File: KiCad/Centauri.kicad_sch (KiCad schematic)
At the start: 137 parts, among them U1 Raspberry_Pi_Pico

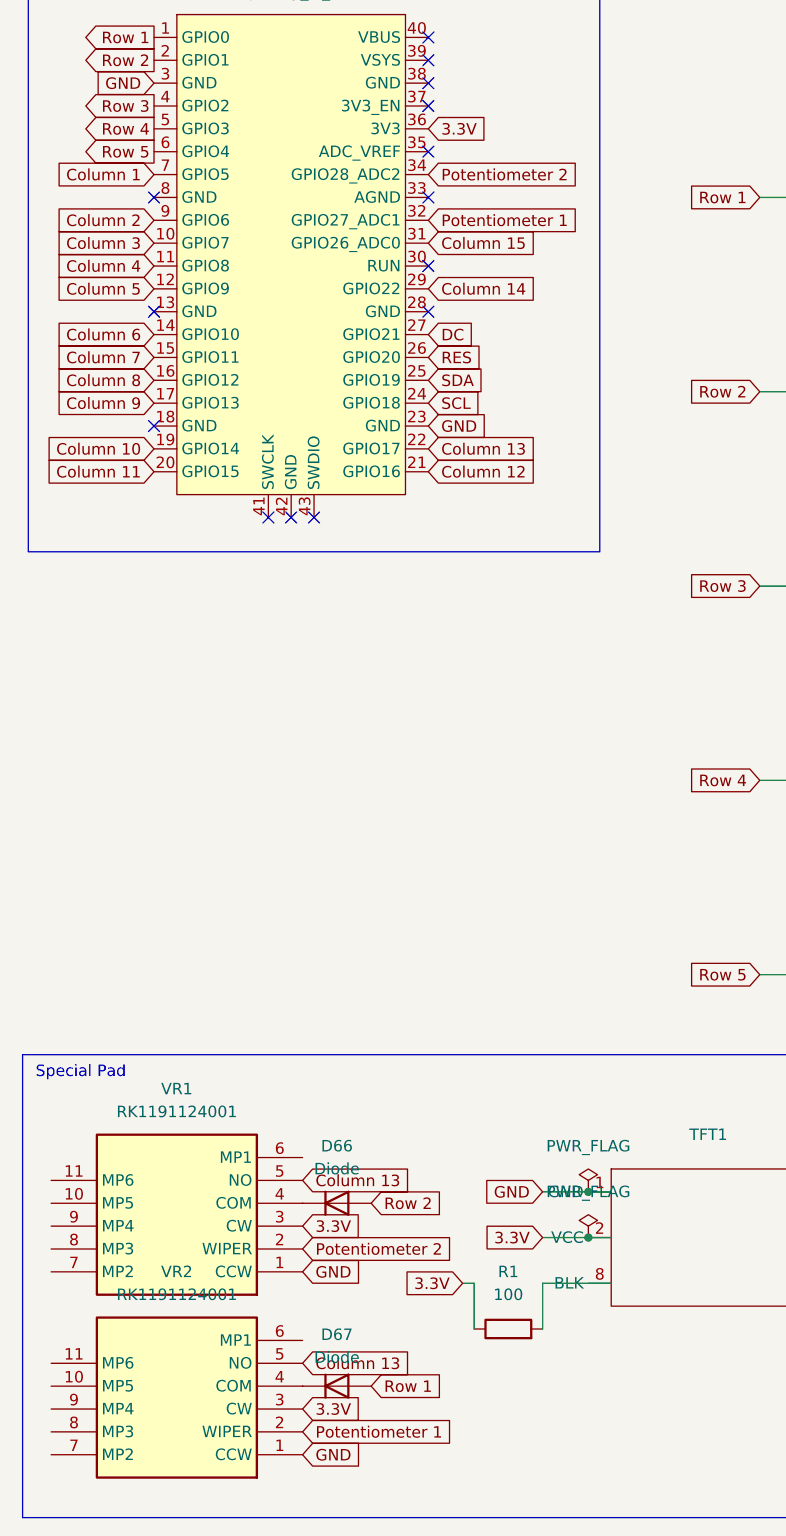
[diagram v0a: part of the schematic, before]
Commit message: Add files via upload
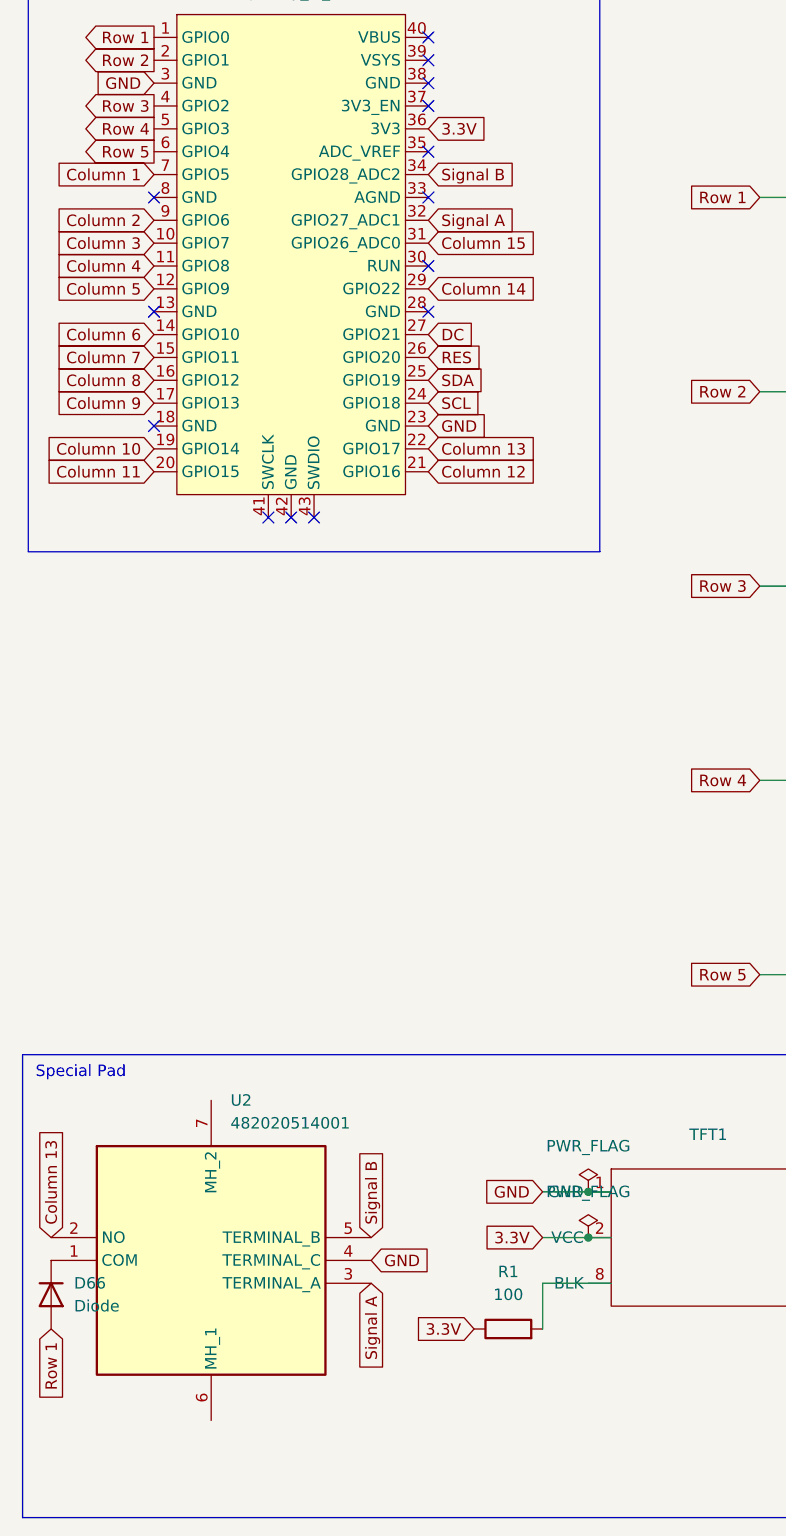
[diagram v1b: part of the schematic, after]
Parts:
- removed D67: Diode, ScottoKeebs_Components:Diode_SOD-123, symbol ScottoKeebs:Placeholder_Diode
- removed VR1, VR2: RK1191124001, RK1191124001:RK1191124001, symbol RK1191124001:RK1191124001
- added U2: 482020514001, 482020514001:482020514001, symbol 482020514001:482020514001
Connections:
- net Column 13: now also U2.2 (NO)
- net GND: now also U2.4 (TERMINAL_C)
- net Row 1: now also D66.2 (A)
- net Row 2: no longer D66.2 (A)
- net at D66.1 (K): now also U2.1 (COM)
- net Potentiometer 1 renamed Signal A
- net Signal A: now also U2.3 (TERMINAL_A)
- net Potentiometer 2 renamed Signal B
- net Signal B: now also U2.5 (TERMINAL_B)
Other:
- moved on the sheet: D66
